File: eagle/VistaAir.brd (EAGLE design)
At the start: 100 x 80 mm, 6 parts

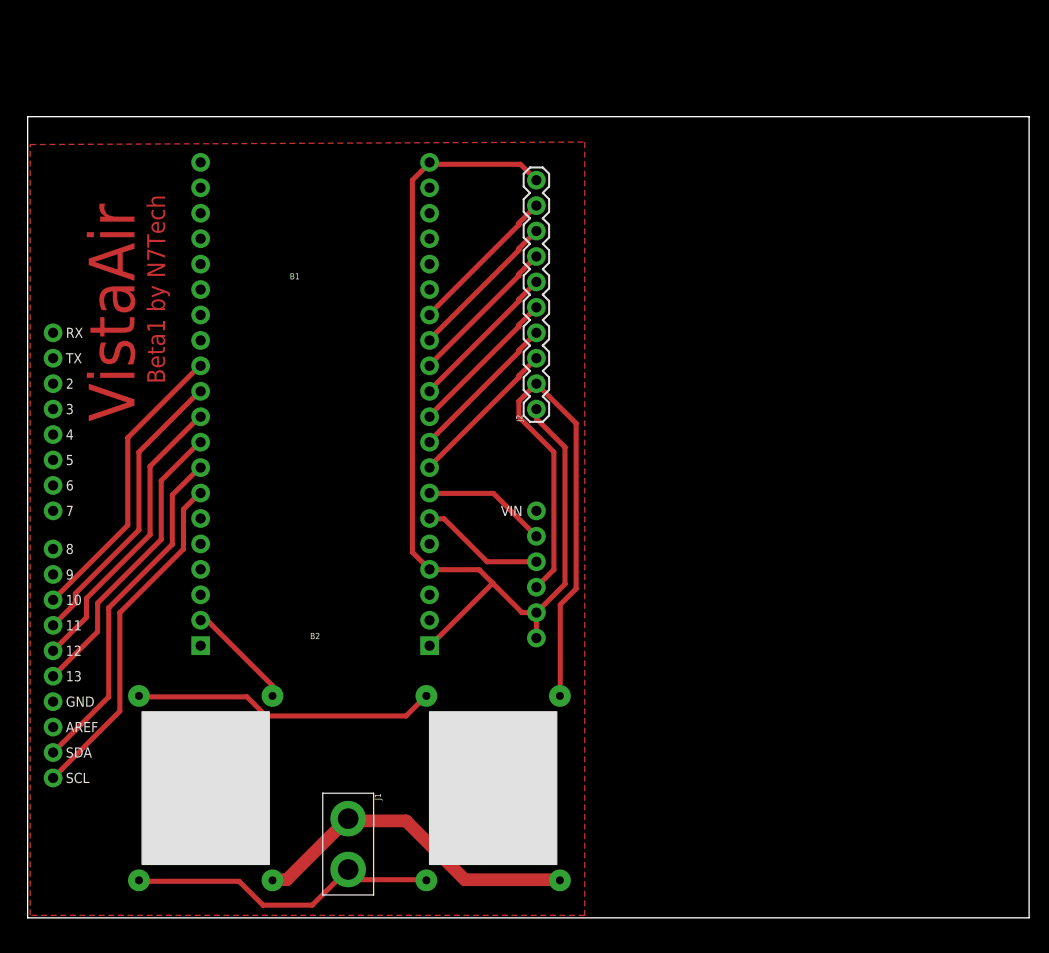
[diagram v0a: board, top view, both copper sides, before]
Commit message: pcb corrections
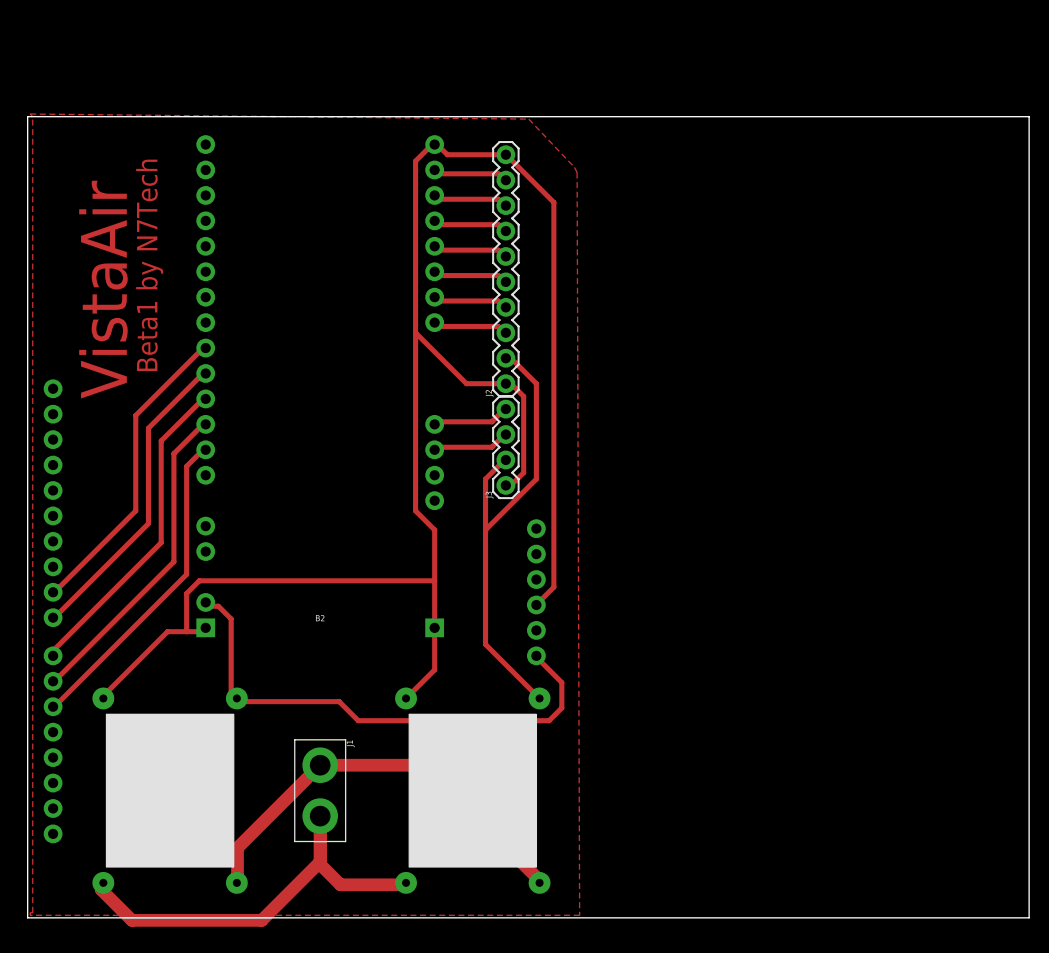
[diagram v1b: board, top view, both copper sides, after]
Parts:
- added J3: (no value), SparkFun-Connectors:1X04
- B2: device SparkFun-Boards:ESP32_THING -> kevins_parts:ESP32_THING
- moved J1 6.02 mm to (29.2, 12.7)
- moved J2 3.97 mm to (47.8, 53.3)
- moved U$1 3.57 mm to (14.2, 12.7)
- moved U$2 2.05 mm to (44.5, 12.7)
- moved B2 1.85 mm to (16.5, 27.7)
- moved B1 0.76 mm to (26.7, 33.8), flipped to the bottom, turned to 180 degrees
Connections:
- removed net GND_OUT: U$1.GND_OUT, U$2.GND_OUT
- removed net LOGIC_V: B2.36
- new net CWL2: B2.7
- new net NC1: B2.35
- new net NC2: B2.34
- net 3V6: now also J3.2; no longer B1.5V
- net BOARD_GND: now also B1.GND@0, B2.1, J3.1, U$1.GND_OUT, U$2.GND_OUT; no longer B1.3.3V, B1.RES, B2.37
- net CCL1: now also B1.D8, B2.11; no longer B1.SDA, B2.8
- net CCL2: now also B1.D9, B2.12; no longer B1.SCL, B2.7
- net CLW1: now also B1.D7, B2.10; no longer B1.D10, B2.12
- net CLW2: now also B1.D4; no longer B1.D13, B2.9
- net ENC1A: now also B2.28; no longer B2.33
- net ENC1B: now also B2.27; no longer B2.32
- net ENC2A: now also B2.33, J3.3; no longer B1.GND@0, B2.35
- net ENC2B: now also B2.32, J3.4; no longer B1.GND@1, B2.34
- net LED: now also B2.22; no longer B2.27
- net LIMBOTA: now also B2.24; no longer B2.29
- net LIMBOTB: now also B2.23; no longer B2.28
- net LIMTOPA: now also B2.26; no longer B2.31
- net LIMTOPB: now also B2.25; no longer B2.30
- net PWM1: now also B1.D5, B2.8; no longer B1.D12, B2.10
- net PWM2: now also B1.D6, B2.9; no longer B1.D11, B2.11
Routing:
- net BOARD_GND: track 100.0 -> 180.0 mm
- net V5IN: track 10.9 -> 52.0 mm
- net GND_OUT: track 30.4 -> 0.00 mm
- net CLW2: track 29.5 -> 0.00 mm
- net GND12: track 33.2 -> 45.2 mm
- net 3V6: track 56.7 -> 47.8 mm
- net V12: track 33.8 -> 42.1 mm
- net ENC1B: track 15.3 -> 7.76 mm
- net ENC1A: track 15.3 -> 7.76 mm
- net LIMTOPB: track 15.3 -> 7.76 mm
- net LIMBOTB: track 15.3 -> 7.76 mm
- net LIMTOPA: track 15.3 -> 7.76 mm
- net LED: track 15.3 -> 7.76 mm
- net LIMBOTA: track 15.3 -> 7.76 mm
- net ENC2B: track 12.5 -> 7.89 mm
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- added copper zone on layer 1, net N$1
- removed copper zone on layer 1, net GND

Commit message: beta 1 board corrections
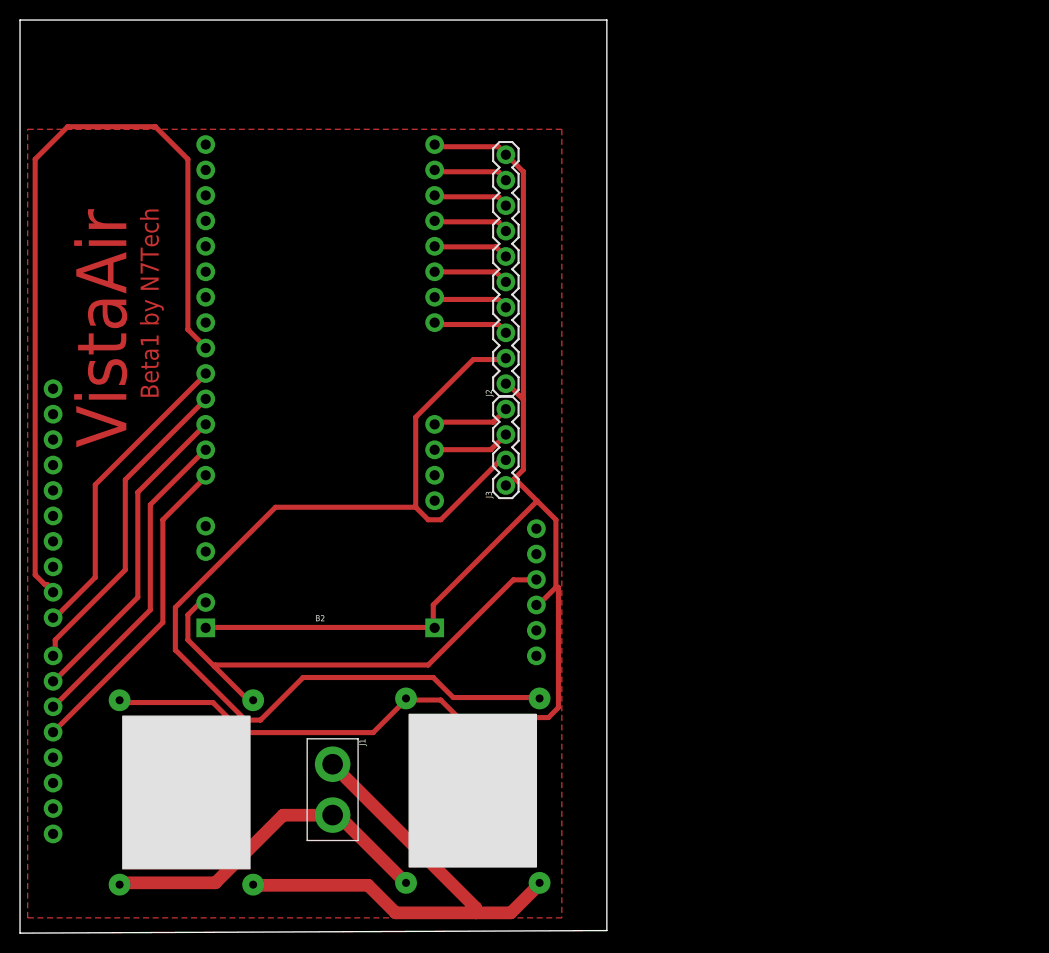
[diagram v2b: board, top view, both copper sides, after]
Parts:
- moved U$1 1.64 mm to (15.8, 12.5)
- moved J1 1.25 mm to (30.5, 12.8)
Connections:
- removed net CWL2: B2.7
- net CLW2: now also B2.7
- net V5IN: now also B1.5V; no longer B1.VIN
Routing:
- net 3V6: track 47.8 -> 106.9 mm
- net CCL2: track 31.6 -> 81.6 mm
- net CLW2: track 0.00 -> 32.0 mm
- net BOARD_GND: track 180.0 -> 159.8 mm
- net GND12: track 45.2 -> 34.3 mm
- net V12: track 42.1 -> 51.8 mm
- net V5IN: track 52.0 -> 49.7 mm
- net PWM2: track 32.8 -> 32.0 mm
- net PWM1: track 32.8 -> 32.0 mm
- net CCL1: track 31.6 -> 30.8 mm
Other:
- board size 100 x 80 mm -> 58.6 x 91.2 mm
